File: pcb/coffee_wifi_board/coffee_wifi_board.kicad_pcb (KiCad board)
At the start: 2 copper layers, 13 parts

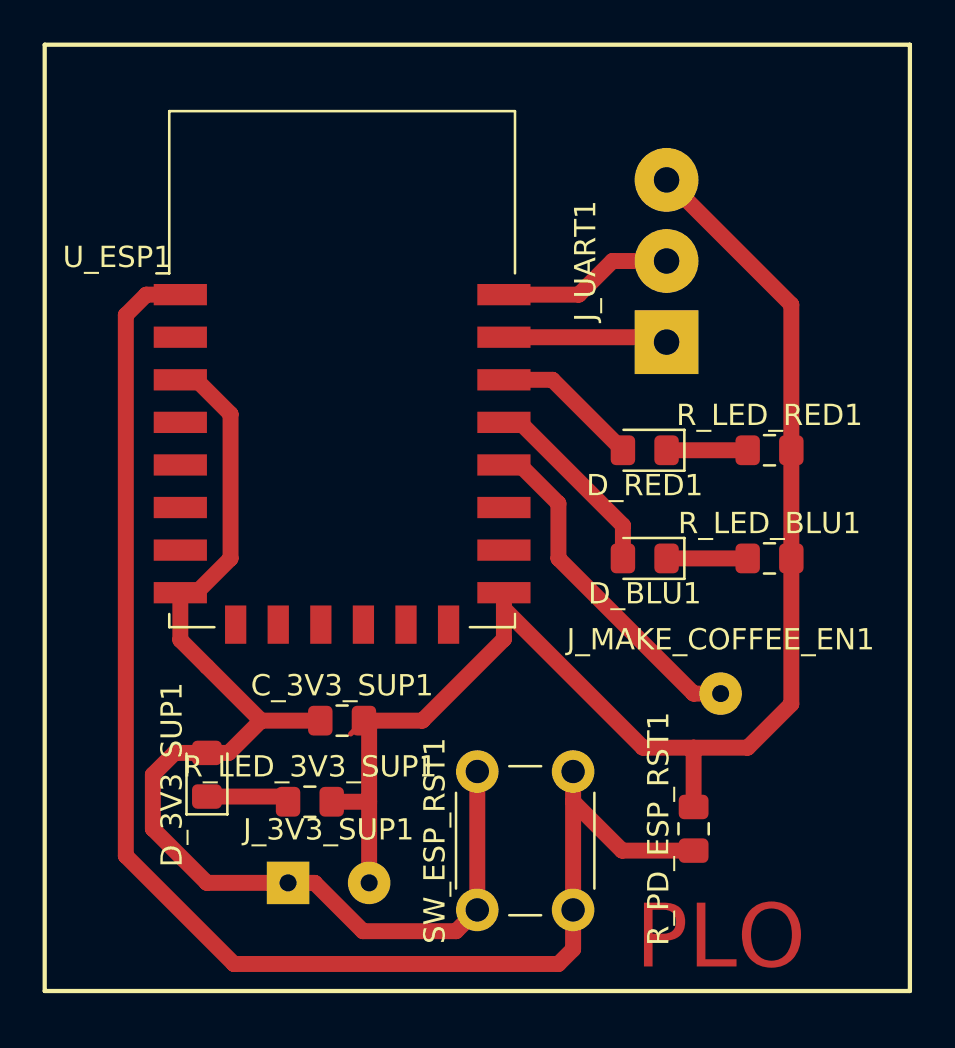
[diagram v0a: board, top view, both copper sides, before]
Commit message: Board rework.
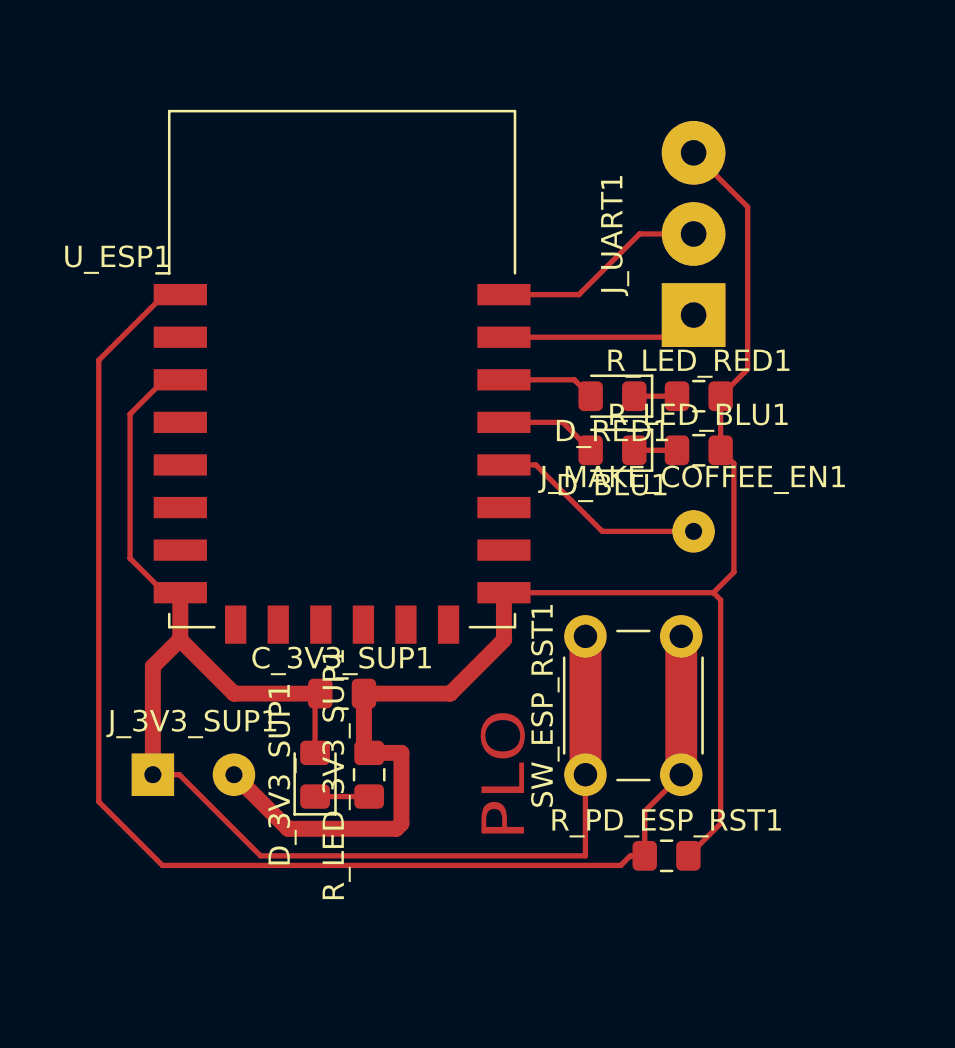
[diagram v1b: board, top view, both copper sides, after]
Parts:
- moved J_3V3_SUP1 8.13 mm to (100.3, 71.1)
- moved SW_ESP_RST1 8.13 mm to (120.7, 71.1)
- moved J_MAKE_COFFEE_EN1 7.73 mm to (125.7, 59.7)
- moved R_LED_BLU1 6.07 mm to (126.0, 55.9)
- moved D_BLU1 5.30 mm to (121.9, 55.9)
- moved D_3V3_SUP1 5.08 mm to (108.0, 71.1)
- moved R_LED_RED1 4.18 mm to (126.0, 53.3)
- moved R_LED_3V3_SUP1 3.06 mm to (110.5, 71.1), turned to 90 degrees
- moved D_RED1 2.96 mm to (121.9, 53.3)
- moved R_PD_ESP_RST1 1.80 mm to (124.5, 74.9), turned to 0 degrees
- moved J_UART1 1.80 mm to (125.7, 49.5)
- moved C_3V3_SUP1 1.27 mm to (109.2, 67.3)
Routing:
- net +3V3: track 56.4 -> 66.2 mm
- net MAKE_COFFEE_EN: track 16.1 -> 10.2 mm
- net LED_BLU: track 9.14 -> 4.62 mm
- net GND: track 69.1 -> 72.5 mm
- net ESP_RST: track 67.0 -> 63.9 mm
- net LED_RED: track 6.96 -> 4.39 mm
- net Net-(D_RED1-Pad1): track 3.81 -> 2.01 mm
- net Net-(D_BLU1-Pad1): track 3.81 -> 2.01 mm
- net UART_TXD: track 8.29 -> 10.1 mm
- net UART_RXD: track 7.74 -> 9.34 mm
- net Net-(D_3V3_SUP1-Pad1): track 3.91 -> 2.54 mm
